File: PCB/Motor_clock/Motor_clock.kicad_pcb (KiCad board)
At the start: 2 copper layers, 111.8 x 73.7 mm, 54 parts, among them J1 WS2812, J10 M_M_2, J11 USB_B_Micro, J2 Barrel_Jack_Switch, J3 Battery_input, J4 ICSP, J5 M_H_1, J6 M_S_1, J7 M_H_1, J8 M_S_2, J9 M_M_1, SW1 DS_reset, SW2 SW_Push, U1 DS3231M, U2 ATmega328P-AU, U3 M_H_1, U4 M_S_1, U5 M_H_2, U6 M_S_2, U7 M_M_1, U8 M_M_2, U9 CH340G, Y1 16Mhz, Y2 12Mhz

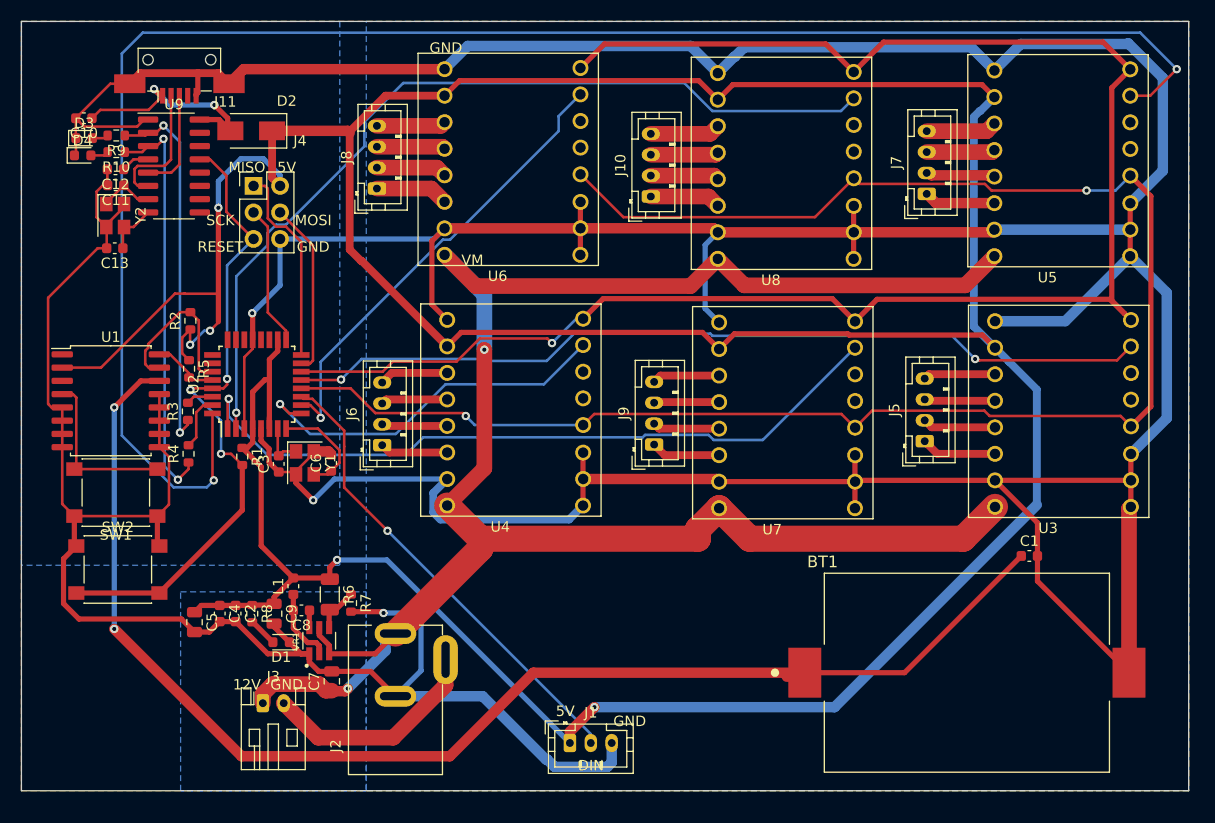
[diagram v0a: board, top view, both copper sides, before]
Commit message: Bug fix
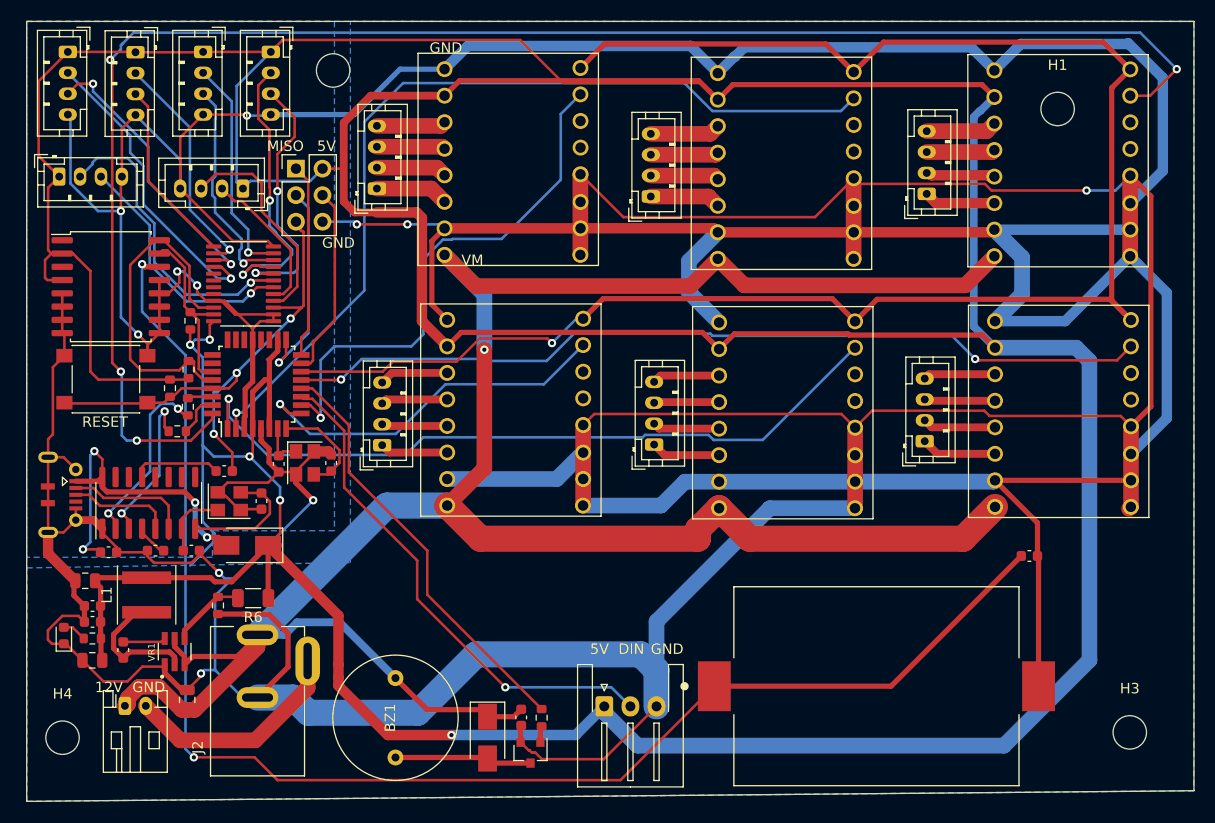
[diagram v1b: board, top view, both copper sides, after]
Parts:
- removed D4: LED, LED_SMD:LED_0603_1608Metric
- removed R10: 1k, Resistor_SMD:R_0603_1608Metric
- removed SW1: DS_reset, Button_Switch_SMD:SW_Push_1P1T_NO_6x6mm_H9.5mm
- added BZ1: Buzzer, Buzzer:buzzer, F.Cu at (145.0, 122.6)
- added C14: 100nF, Capacitor_SMD:C_0603_1608Metric, F.Cu at (128.6, 98.9)
- added C15: 100nF, Capacitor_SMD:C_0603_1608Metric, F.Cu at (157.1, 122.5)
- added G***: LOGO, picture:logo, B.Cu at (202.7, 116.3)
- added H1: MountingHole, MountingHole:MountingHole_3.2mm_M3, F.Cu at (208.4, 64.3)
- added H2: MountingHole, MountingHole:MountingHole_3.2mm_M3, F.Cu at (139.1, 60.6)
- added H3: MountingHole, MountingHole:MountingHole_3.2mm_M3, F.Cu at (215.3, 124.0)
- added H4: MountingHole, MountingHole:MountingHole_3.2mm_M3, F.Cu at (113.2, 124.5)
- added J12: Enc_M_2, Connector_JST:JST_PH_B4B-PH-K_1x04_P2.00mm_Vertical, F.Cu at (133.1, 58.8)
- added J13: Enc_H_2, Connector_JST:JST_PH_B4B-PH-K_1x04_P2.00mm_Vertical, F.Cu at (120.1, 58.8)
- added J14: Enc_S_2, Connector_JST:JST_PH_B4B-PH-K_1x04_P2.00mm_Vertical, F.Cu at (130.4, 71.9)
- added J15: Enc_S_1, Connector_JST:JST_PH_B4B-PH-K_1x04_P2.00mm_Vertical, F.Cu at (112.8, 70.7)
- added J16: Enc_M1, Connector_JST:JST_PH_B4B-PH-K_1x04_P2.00mm_Vertical, F.Cu at (126.6, 58.8)
- added J17: Enc_H_1, Connector_JST:JST_PH_B4B-PH-K_1x04_P2.00mm_Vertical, F.Cu at (113.7, 58.8)
- added Q1: Q_NPN_BEC, Package_TO_SOT_SMD:SOT-23, F.Cu at (158.0, 125.9)
- added U10: TCA9548APWR, Package_SO:TSSOP-24_4.4x7.8mm_P0.65mm, F.Cu at (130.5, 81.0)
- D3: value LED -> 1N5819; footprint LED_SMD:LED_0603_1608Metric -> Diode_SMD:D_SMA
- J1: footprint Connector_JST:JST_PH_B3B-PH-K_1x03_P2.00mm_Vertical -> Connector_JST:JST_XH_S3B-XH-A-1_1x03_P2.50mm_Horizontal
- J11: footprint Connector_USB:USB_Mini-B_AdamTech_MUSB-B5-S-VT-TSMT-1_SMD_Vertical -> USB:MicroXNJ
- L1: footprint Inductor_SMD:L_0603_1608Metric -> Inductor_SMD:L_Coilcraft_XAL5030
- moved D3 69.2 mm to (153.8, 124.5), turned to 270 degrees
- moved R9 69.0 mm to (159.0, 122.5), turned to 90 degrees
- moved C10 41.6 mm to (117.6, 106.7), turned to 0 degrees
- moved J11 41.0 mm to (114.4, 101.2), turned to 270 degrees
- moved D2 39.7 mm to (130.8, 106.0)
- moved C12 36.7 mm to (122.1, 106.6)
- moved C11 35.7 mm to (125.5, 106.6), turned to 0 degrees
- moved U9 32.3 mm to (121.4, 102.0), turned to 90 degrees
- moved Y2 29.4 mm to (129.1, 101.8), turned to 0 degrees
- moved C13 28.0 mm to (132.2, 101.8), turned to 270 degrees
- moved D1 20.8 mm to (113.3, 114.7), turned to 90 degrees
- moved SW2 18.3 mm to (117.3, 90.1)
- moved C9 18.0 mm to (116.0, 117.1), turned to 180 degrees
- moved C8 17.5 mm to (119.0, 116.1), turned to 270 degrees
- moved R8 15.5 mm to (116.0, 115.0), turned to 180 degrees
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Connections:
- BT1 pad 2: GND -> PDN
- C1 pad 2: GND -> PDN
- C10 pad 2: GND -> PDN
- C11 pad 2: GND -> PDN
- C12 pad 2: GND -> PDN
- C13 pad 2: GND -> PDN
- C2 pad 2: GND -> PDN
- C3 pad 1: GND -> PDN
- C4 pad 2: GND -> PDN
- C5 pad 2: GND -> PDN
- C6 pad 2: GND -> PDN
- C7 pad 2: GND -> PDN
- C9 pad 2: GND -> PDN
- D1 pad 1: GND -> PDN
- D3 pad 1: GND -> 12V
- D3 pad 2: Net-(D3-Pad2) -> Net-(BZ1-Pad2)
- J1 pad 3: GND -> PDN
- J11 pad 5: GND -> PDN
- J11 pad 6: GND -> PDN
- J2 pad 3: GND -> PDN
- J4 pad 6: GND -> PDN
- R7 pad 2: GND -> PDN
- R9 pad 1: TX -> Net-(Q1-Pad1)
- R9 pad 2: Net-(D3-Pad2) -> Buzzer
- SW2 pad 1: GND -> PDN
- U1 pad 10: GND -> PDN
- U1 pad 11: GND -> PDN
- U1 pad 12: GND -> PDN
- U1 pad 13: GND -> PDN
- U1 pad 4: Net-(SW1-Pad2) -> +5V
- U1 pad 5: GND -> PDN
- U1 pad 6: GND -> PDN
- U1 pad 7: GND -> PDN
- U1 pad 8: GND -> PDN
- U1 pad 9: GND -> PDN
- U2 pad 12: PDN -> Buzzer
- U2 pad 21: GND -> PDN
- U2 pad 3: GND -> PDN
- U2 pad 5: GND -> PDN
- U3 pad 1: GND -> PDN
- U3 pad 10: GND -> PDN
- U3 pad 16: GND -> PDN
- U3 pad 2: GND -> PDN
- U3 pad 3: GND -> PDN
- U4 pad 1: GND -> PDN
- U4 pad 10: GND -> PDN
- U4 pad 16: GND -> PDN
- U4 pad 2: GND -> PDN
- U4 pad 3: GND -> PDN
- U5 pad 1: GND -> PDN
- U5 pad 10: GND -> PDN
- U5 pad 16: GND -> PDN
- U5 pad 2: GND -> PDN
- U5 pad 3: GND -> PDN
- U6 pad 1: GND -> PDN
- U6 pad 10: GND -> PDN
- U6 pad 16: GND -> PDN
- U6 pad 2: GND -> PDN
- U6 pad 3: GND -> PDN
- U7 pad 1: GND -> PDN
- U7 pad 10: GND -> PDN
- U7 pad 16: GND -> PDN
- U7 pad 2: GND -> PDN
- U7 pad 3: GND -> PDN
- U8 pad 1: GND -> PDN
- U8 pad 10: GND -> PDN
- U8 pad 16: GND -> PDN
- U8 pad 2: GND -> PDN
- U8 pad 3: GND -> PDN
- U9 pad 1: GND -> PDN
- U9 pad 13: RESET -> Net-(C14-Pad1)
- VR1 pad 1: GND -> PDN
- Y1 pad 2: GND -> PDN
- Y1 pad 4: GND -> PDN
- Y2 pad 2: GND -> PDN
- Y2 pad 4: GND -> PDN
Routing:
- net PDN: track 165.7 -> 929.8 mm, vias 2 -> 11
- net GND: track 627.5 -> 0.00 mm, vias 3 -> 0
- net +5V: track 382.8 -> 544.5 mm
- net 12V: track 182.1 -> 224.7 mm, vias 2 -> 1
- net Buzzer: track 0.00 -> 40.9 mm
- net SC1: track 0.00 -> 29.7 mm, vias 0 -> 1
- net SC5: track 0.00 -> 29.2 mm, vias 0 -> 1
- net SC2: track 0.00 -> 28.1 mm, vias 0 -> 2
- net SD5: track 0.00 -> 27.4 mm, vias 0 -> 2
- net SCL: track 6.98 -> 32.8 mm
- net SD2: track 0.00 -> 25.1 mm, vias 0 -> 2
- net SD1: track 0.00 -> 24.2 mm, vias 0 -> 1
- net RX: track 39.7 -> 15.6 mm
- net SC4: track 0.00 -> 22.3 mm, vias 0 -> 1
- net SC3: track 0.00 -> 21.4 mm, vias 0 -> 1
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- added copper zone on B.Cu, net PDN
- removed copper zone on B.Cu, net GND
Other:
- board size 111.8 x 73.7 mm -> 111.8 x 74.7 mm
- board text added: "+"
- board text added: "H_1"
- board text added: "H_2"
- board text added: "M_1"
- board text added: "M_2"
- board text added: "S_1"
- board text added: "S_2"
- board text removed: "MOSI"
- board text removed: "SCK"
